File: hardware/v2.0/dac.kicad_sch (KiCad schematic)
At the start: 4 parts, among them IC3 LTC2630ISC6-LZ12#TRMPBF, J8 530480210, U1 ECP5U-25F-CABGA256

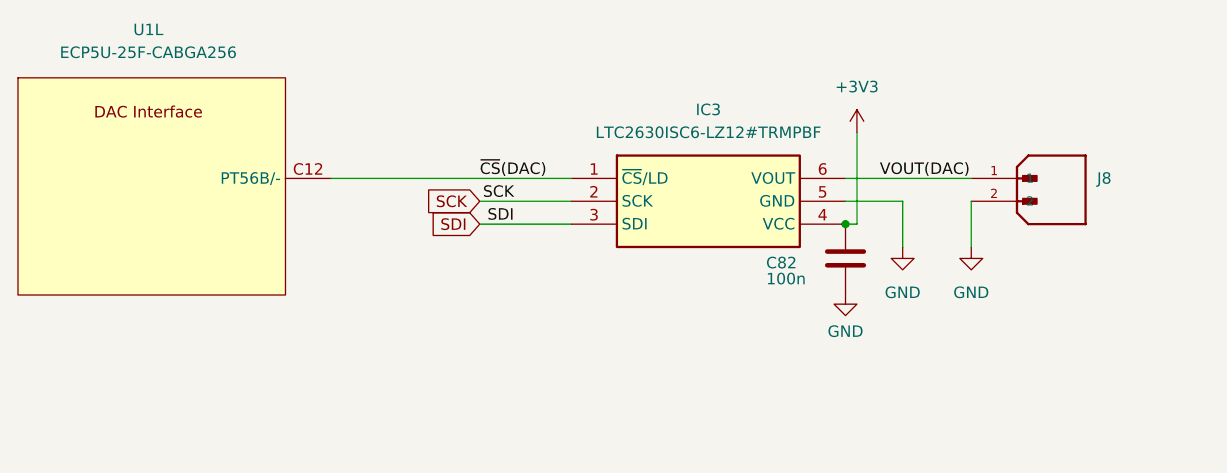
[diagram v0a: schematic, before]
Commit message: 2CH DAC
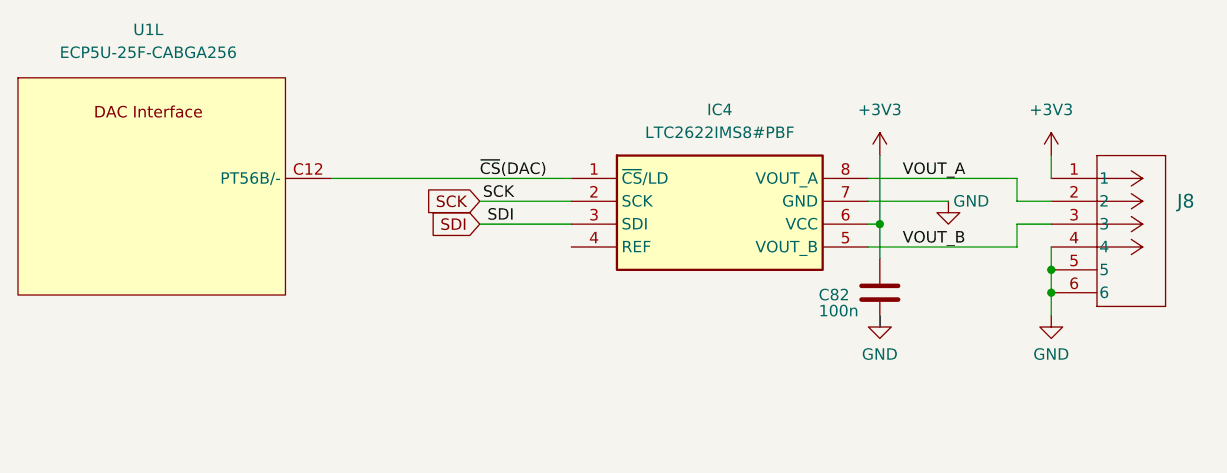
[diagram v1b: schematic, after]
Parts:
- removed IC3: LTC2630ISC6-LZ12#TRMPBF, SOT65P210X100-6N, symbol LTC2630ISC6-LZ12#TRMPBF:LTC2630ISC6-LZ12#TRMPBF
- removed J8: 530480210, 530480210:MOLEX_530480210, symbol 530480210:530480210
- added IC4: LTC2622IMS8#PBF, SOP65P490X110-8N, symbol LTC2622IMS8#PBF:LTC2622IMS8#PBF
- added J8: BM04B-ACHSS-A-GAN-TFLFSN, CONN_BM04B-ACHSS-A-GAN-TFLFSN_JST, symbol BM04B_ACHSS_A_GAN_TF_LF__SN:BM04B-ACHSS-A-GAN-TFLFSN
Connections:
- net +3V3: now also IC4.6 (VCC), J8.1
- net GND: now also IC4.7 (GND), J8.4, J8.5, J8.6
- net SCK: now also IC4.2 (SCK)
- net SDI: now also IC4.3 (SDI)
- net ~{CS}(DAC): now also IC4.1 (~{CS}/LD)
- new net VOUT_A: IC4.8 (VOUT_A), J8.2
- new net VOUT_B: IC4.5 (VOUT_B), J8.3
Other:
- moved on the sheet: C82
